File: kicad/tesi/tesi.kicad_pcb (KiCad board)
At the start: 2 copper layers, 100 x 100 mm, 35 parts, among them J1 Conn_01x02_Socket, J2 Conn_01x06_Socket, SW1 POWER, U1 MAX4466, U2 BNO055, U3 MPR121, U4 VL53L1CX

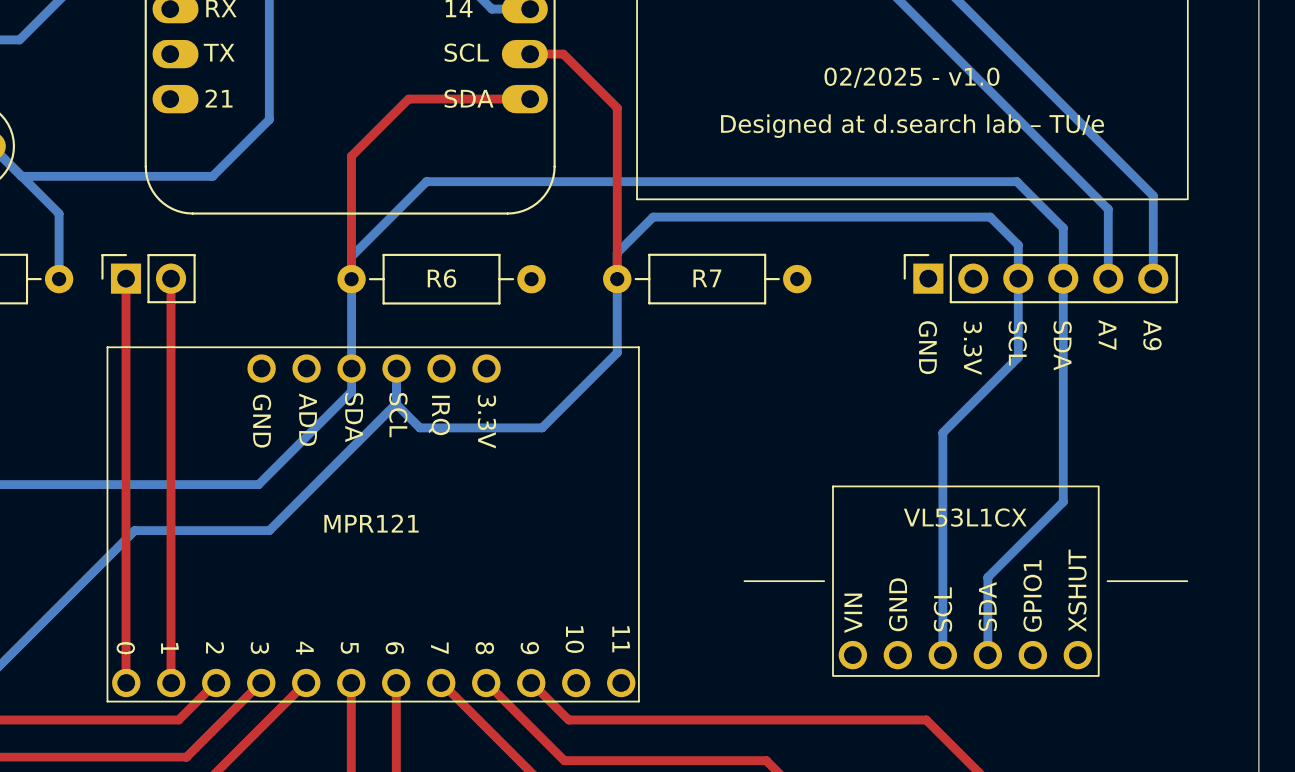
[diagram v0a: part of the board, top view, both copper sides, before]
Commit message: update for submission
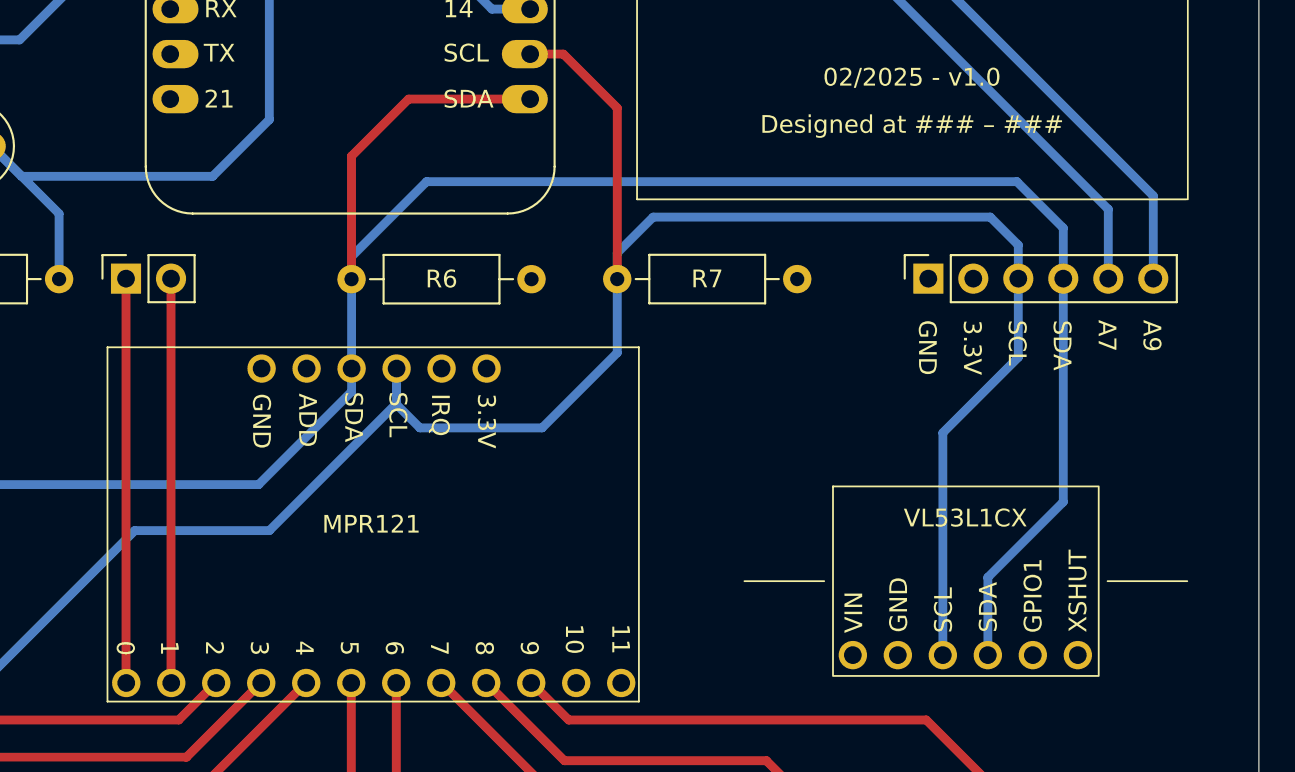
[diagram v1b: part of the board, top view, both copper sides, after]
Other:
- board text added: "Designed at ### – ###"
- board text removed: "Designed at d.search lab – TU/e"

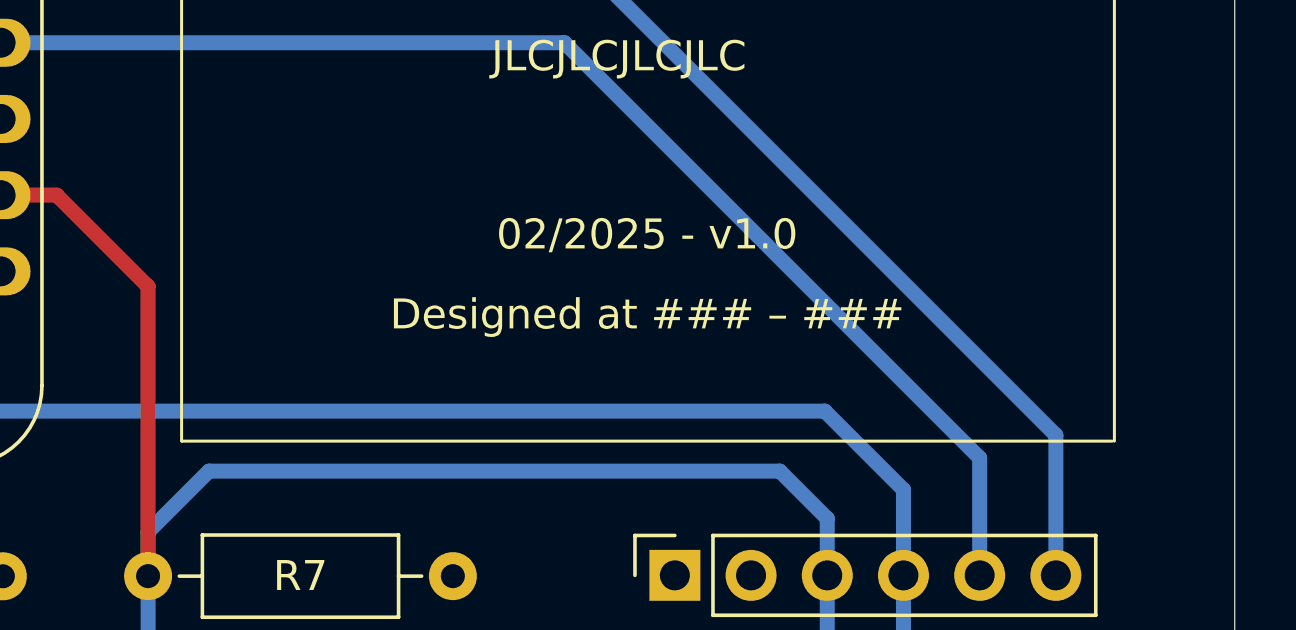
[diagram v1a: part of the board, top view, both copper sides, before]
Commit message: add kicad files
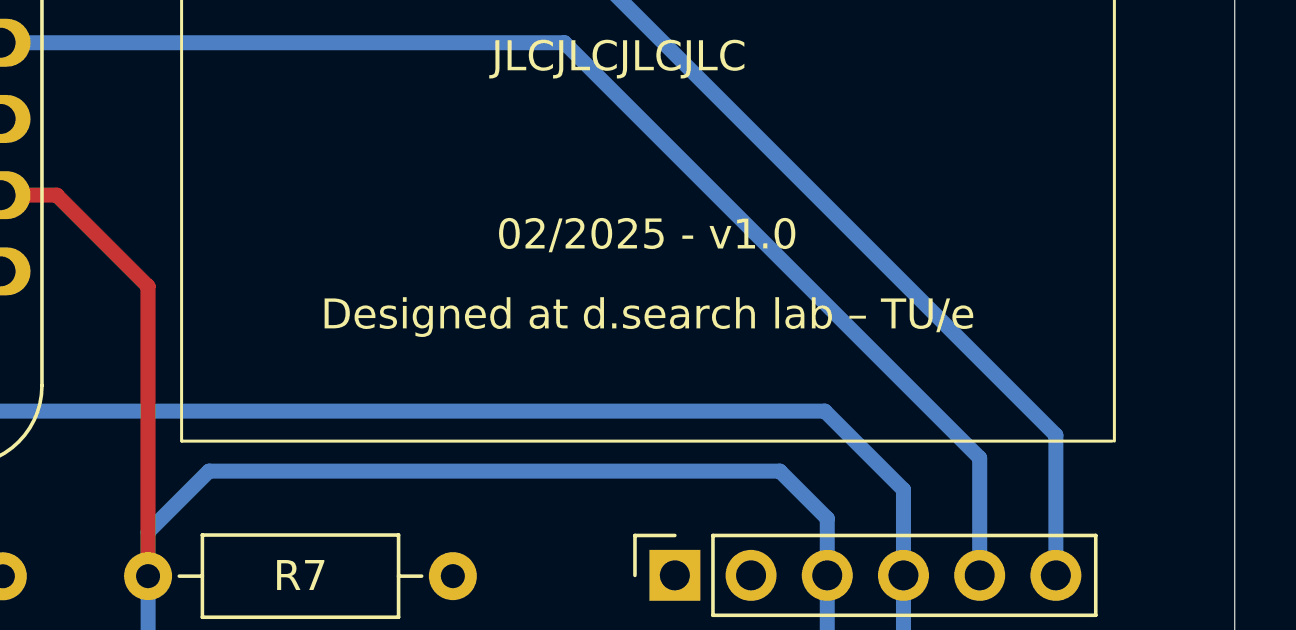
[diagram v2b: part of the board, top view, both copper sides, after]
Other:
- board text added: "Designed at d.search lab – TU/e"
- board text removed: "Designed at ### – ###"
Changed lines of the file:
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@@
 		)
 	)
-	(gr_text "Designed at ### – ###"
-		(at 131.07758 81.36571 0)
+	(gr_text "Designed at d.search lab – TU/e"
+		(at 131.10446 81.36571 0)
 		(layer "F.SilkS")
 		(effects
